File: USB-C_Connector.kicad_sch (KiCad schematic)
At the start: 6 parts, among them J6 USB_C_Receptacle_USB2.0_16P

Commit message: final schem is done
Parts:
- C20: footprint Capacitor_SMD:C_0805_2012Metric -> Capacitor_SMD:C_0805_2012Metric_Pad1.18x1.45mm_HandSolder
- D10: Mouser Part Number 576-SP0503BAHTG -> (none)
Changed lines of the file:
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@@
-			)
-		)
-		(property "Mouser Part Number" "576-SP0503BAHTG "
-			(at 77.4198 81.7763 0)
-			(hide yes)
-			(show_name no)
-			(do_not_autoplace no)
-			(effects
-				(font
-					(size 1.27 1.27)
-				)
 			)
 		)
@@
 			)
 		)
-		(property "Footprint" "Capacitor_SMD:C_0805_2012Metric"
+		(property "Footprint" "Capacitor_SMD:C_0805_2012Metric_Pad1.18x1.45mm_HandSolder"
 			(at 61.2146 33.5163 0)
 			(hide yes)
@@
 		)
 	)
-	(group "USB-C_Connector"
-		(lib_id "LHRS_Design_Blocks:USB-C_Connector")
-		(members "04fcef97-89c4-4537-93b4-3c86159ab421" "0727745f-19bf-4925-85c4-dd8f7685525d"
-			"0c6766ab-f5e4-4ea1-aa18-b77d4fb016d9" "10f106ca-d900-4670-b207-c9eb3ed23f0b"
-			"11166e4d-ed43-481f-b5d0-bf4780e18aa9" "1574fbd0-4d82-4f5b-b7fc-72523f779461"
-			"1930a8c6-0dbc-4b73-84c9-9e39e936dff7" "1be4ba29-309d-4466-aa64-bd1c3c9fb213"
-			"1c6676d9-655e-47b0-993b-851f93b29be0" "1e4802a2-1696-4f84-a997-10989ac104a8"
-			"1f25a7a1-3996-4447-8050-4b3ac7a95bf9" "1fe3fa78-8c96-4fec-92a4-65d0f069d53a"
-			"22e3b80d-58af-4dbf-a1b7-78f5a2f207aa" "23158f13-92ad-4941-93b0-f1b8cff4aef4"
-			"2a48ed1f-dc7d-4c38-bbcc-b1417c5f4741" "2b7acb43-51eb-4fa4-9f12-1927ee42daf1"
-			"31c1c8b0-f199-43b5-8a72-395cd877a32e" "33f91bc2-235d-4c59-8c12-7fb804a19a6f"
-			"38cfcb3e-cf11-4d3d-b993-b5e9d40c61db" "3dd8b24a-ee6e-4824-9390-9c9f75b69509"
-			"4d9e1693-38c4-48c2-97ae-99445c572898" "5267cea2-22b6-4dd5-b54b-587e459b53db"
-			"54d253f2-7913-42ba-ad0d-7fd8d87d8c1a" "55ebce0d-f91e-4ae9-a250-6b724ee2f0e7"
-			"5cb5db20-c658-4655-b1f8-be4d049dfe5d" "5df1d662-b892-424e-ad96-12cc856e36bc"
-			"5f8ebd46-e768-42a2-8166-0ebf166f18c1" "65186f5e-89c9-40b3-814d-2cf851585342"
-			"65336ee7-49d4-4f3a-a16f-d1f78edab5fe" "68179028-fd32-48bf-b395-75eff4b0affa"
-			"728034de-1f4f-43c4-b764-799f66fbad77" "7efbf9ae-a4bd-411a-bd4f-73e22aa56aa3"
-			"87665ee5-842f-4ab8-b4ef-f09e77cb2a70" "8b7605fe-b6c6-4d30-93a4-c62c835ad448"
-			"8c836a32-9398-46ee-a6a0-aaffb1454707" "8e96c2fd-ebbf-4b3c-8059-00ac1477b0f5"
-			"9075ed5e-cbfb-486f-b1fc-3da50c5cd78a" "90e8ec2f-5095-48d1-819b-b485cf0227c1"
-			"97558857-315f-4441-9f30-523800dc3185" "98c5750f-70e6-4fa2-8eb9-777cf9081d1e"
-			"a0373b3d-e712-493b-b572-5da529970808" "a1333329-f4e2-40f5-9812-35a41f66040e"
-			"a81e821b-87aa-475b-bf58-767a3467050c" "b55e0efa-0cd1-43ab-ab03-928614063bd2"
-			"b6c62b86-d9aa-427b-880f-12480ba24203" "b89dd526-8205-4c51-a632-c4e8f4251bd1"
-			"bb253572-93fa-4369-bbf7-5f45d193f6ff" "c072b2d4-24ef-4397-8af9-5c401c4916c0"
-			"c2ea544c-0d4a-4c83-a51a-44bd5212c87e" "c3a8983e-39ad-4f32-83a9-160df684dd0a"
-			"c9339f37-f006-4dc3-be37-72e28a4df71e" "cd1c2b74-2fcc-404c-94d7-1e57e98b6cfa"
-			"d3989971-ceab-4208-a34b-81b2d047226d" "da76b70d-1d08-42fa-9779-e2d100318d24"
-			"ddd5b2e9-7de5-4c9f-ae2c-dd8ab09fd01e" "e879a343-4040-44ca-859b-5c53011819aa"
-			"f4c3dd7f-84ec-4dcb-899f-0b4a41d3690f" "f4ec8c7e-18bb-4be1-a89d-65ff20130820"
-			"f534bb3b-6b47-4793-bfca-fc1faeca945d" "f5ff9e18-5e74-4d5f-8fdc-2ac8288475eb"
-			"f870526d-8e11-4cdd-9f5e-df7546f56408" "f9f29e46-bcf2-4cdd-8cbd-013cb79f55a6"
-		)
-	)

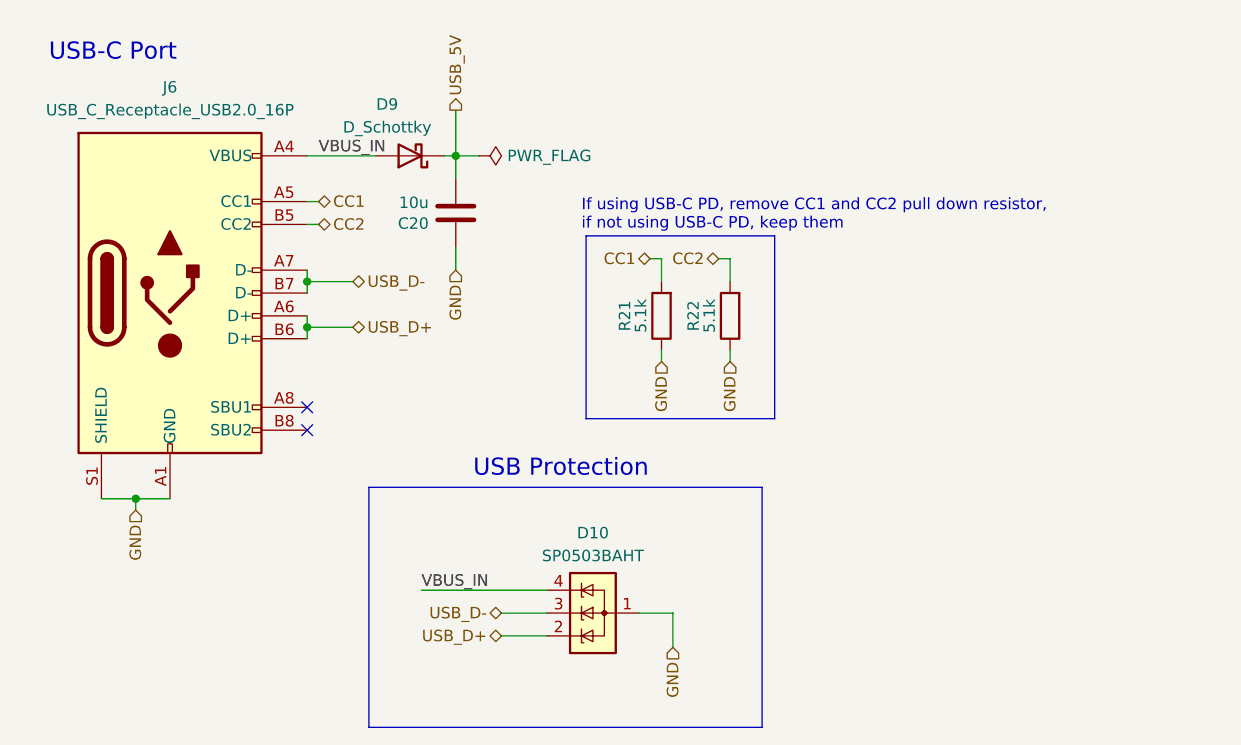
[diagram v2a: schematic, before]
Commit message: shoupu review done
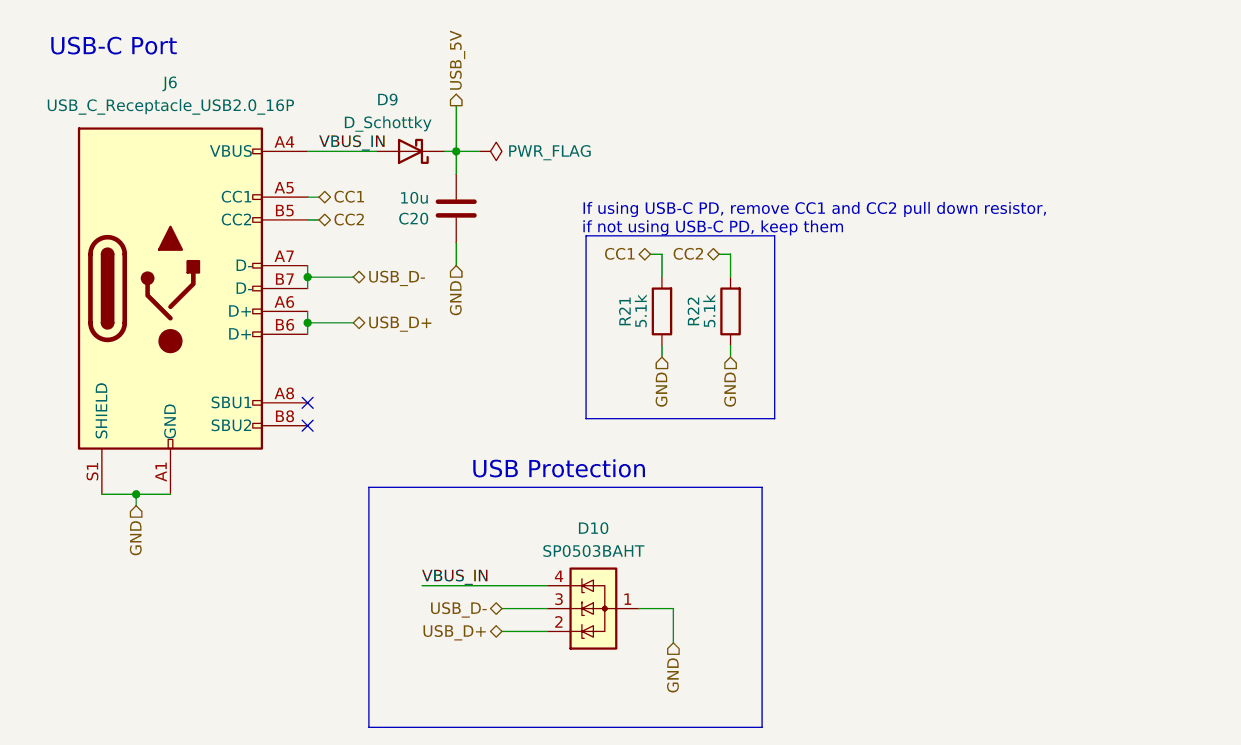
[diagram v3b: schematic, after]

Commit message: review council
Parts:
- J6: footprint LHRS_ICs:USB_C_Receptacle_GCT_USB4105-xx-A_16P_TopMnt_Horizontal -> LHRS_Connectors:USB_C_Receptacle_GCT_USB4105-xx-A_16P_TopMnt_Horizontal
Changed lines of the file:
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@@
 			)
 		)
-		(property "Footprint" "LHRS_ICs:USB_C_Receptacle_GCT_USB4105-xx-A_16P_TopMnt_Horizontal"
+		(property "Footprint" "LHRS_Connectors:USB_C_Receptacle_GCT_USB4105-xx-A_16P_TopMnt_Horizontal"
 			(at 34.29 45.72 0)
 			(hide yes)
